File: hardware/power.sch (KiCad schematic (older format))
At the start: 49 parts, among them J4 USB_C_Receptacle, J5 Conn_01x01, J6 Conn_01x01, U10 TLV62568DBV, U2 TP4056, U4 XC6206P302MR, U7 TLV62568DBV, U8 TLV62568DBV, U9 TLV62568DBV

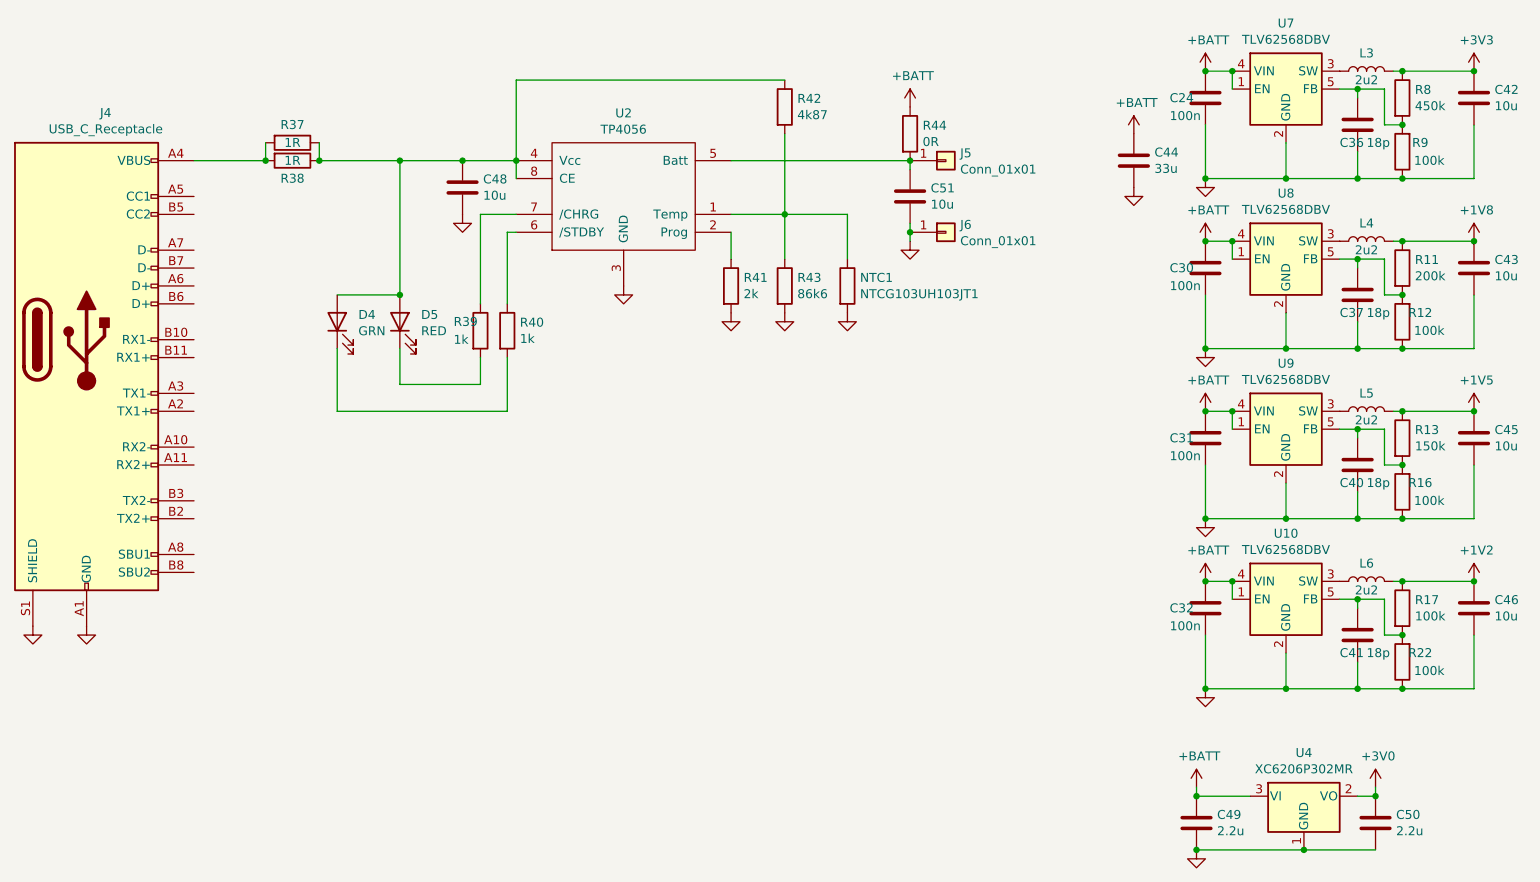
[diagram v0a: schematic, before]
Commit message: Power routing done
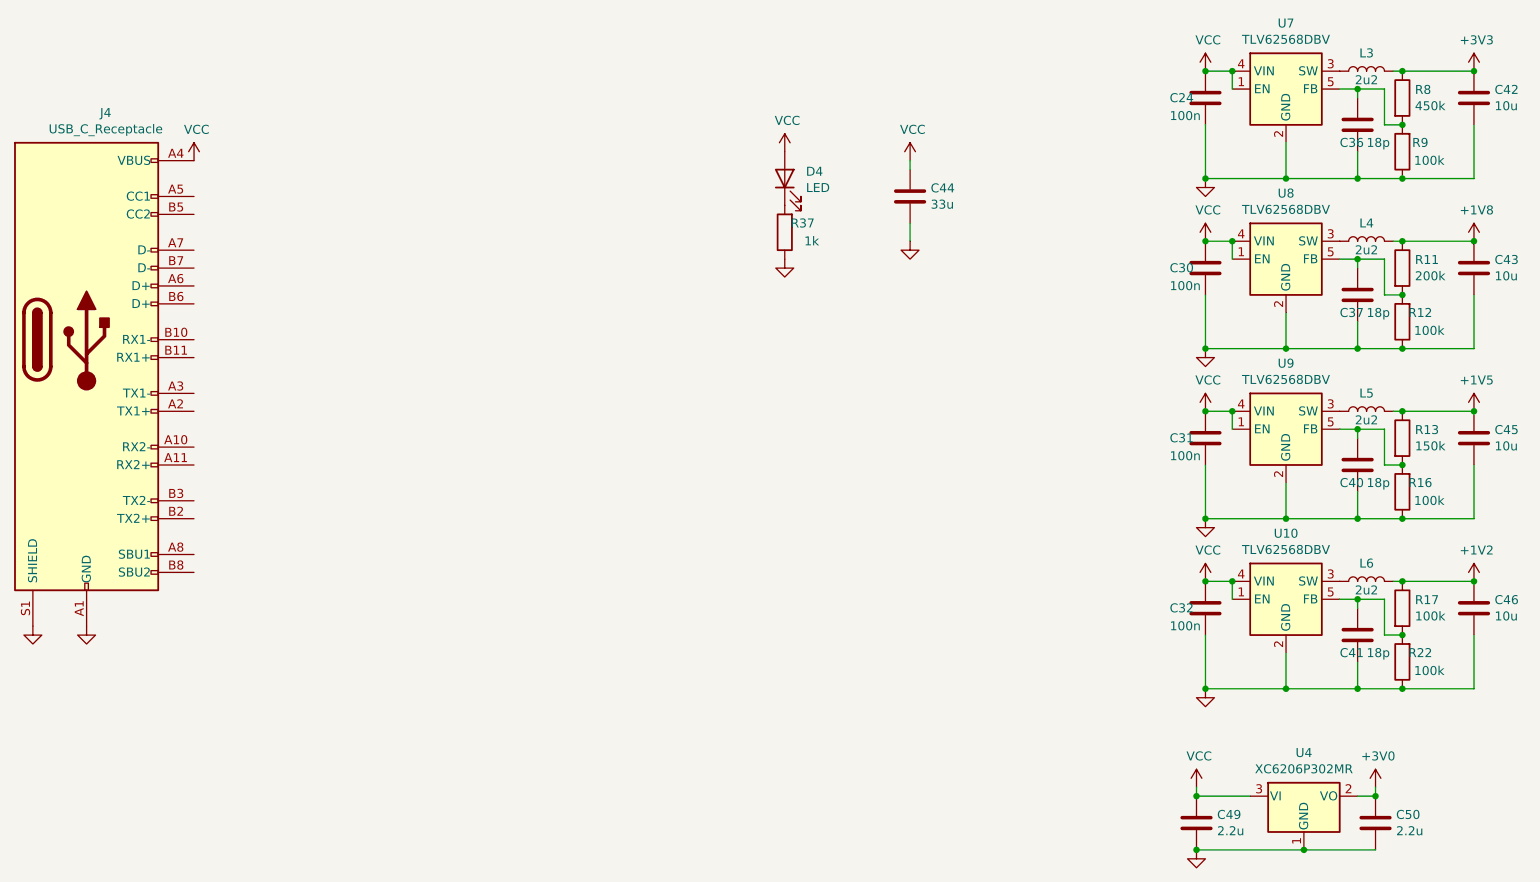
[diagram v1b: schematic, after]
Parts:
- removed C48, C51: 10u, Capacitor_SMD:C_0805_2012Metric, symbol Device:C
- removed D5: RED, LED_SMD:LED_0603_1608Metric, symbol Device:LED
- removed J5, J6: Conn_01x01, TestPoint:TestPoint_THTPad_1.0x1.0mm_Drill0.5mm, symbol Connector_Generic:Conn_01x01
- removed NTC1: NTCG103UH103JT1, Resistor_SMD:R_0603_1608Metric, symbol Device:R
- removed R38: 1R, Resistor_SMD:R_0603_1608Metric, symbol Device:R
- removed R39, R40: 1k, Resistor_SMD:R_0603_1608Metric, symbol Device:R
- removed R41: 2k, Resistor_SMD:R_0603_1608Metric, symbol Device:R
- removed R42: 4k87, Resistor_SMD:R_0603_1608Metric, symbol Device:R
- removed R43: 86k6, Resistor_SMD:R_0603_1608Metric, symbol Device:R
- removed R44: 0R, Resistor_SMD:R_0603_1608Metric, symbol Device:R
- removed U2: TP4056, Package_SO:SOP-8_3.9x4.9mm_P1.27mm, symbol custom:TP4056
- D4: value GRN -> LED
- R37: value 1R -> 1k
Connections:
- net +BATT is gone; now on net VCC: C24.1, C30.1, C31.1, C32.1, C44.1, C49.1, U10.1 (EN), U10.4 (VIN), U4.3 (VI), U7.1 (EN), U7.4 (VIN), U8.1 (EN), U8.4 (VIN), U9.1 (EN), U9.4 (VIN)
- net GND: now also R37.1
- net VCC: now reaches D4.2 (A)
- net VCC: now also J4.A4 (VBUS), J4.A9 (VBUS), J4.B4 (VBUS), J4.B9 (VBUS); no longer R37.1
- net at D4.1 (K): now also R37.2
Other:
- moved on the sheet: C44

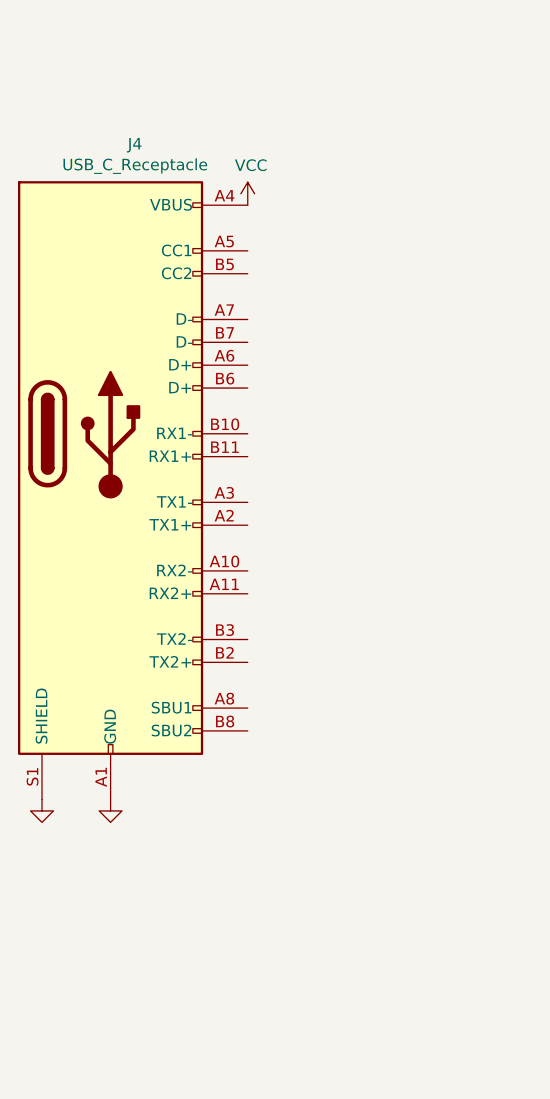
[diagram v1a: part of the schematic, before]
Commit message: Small touch-ups
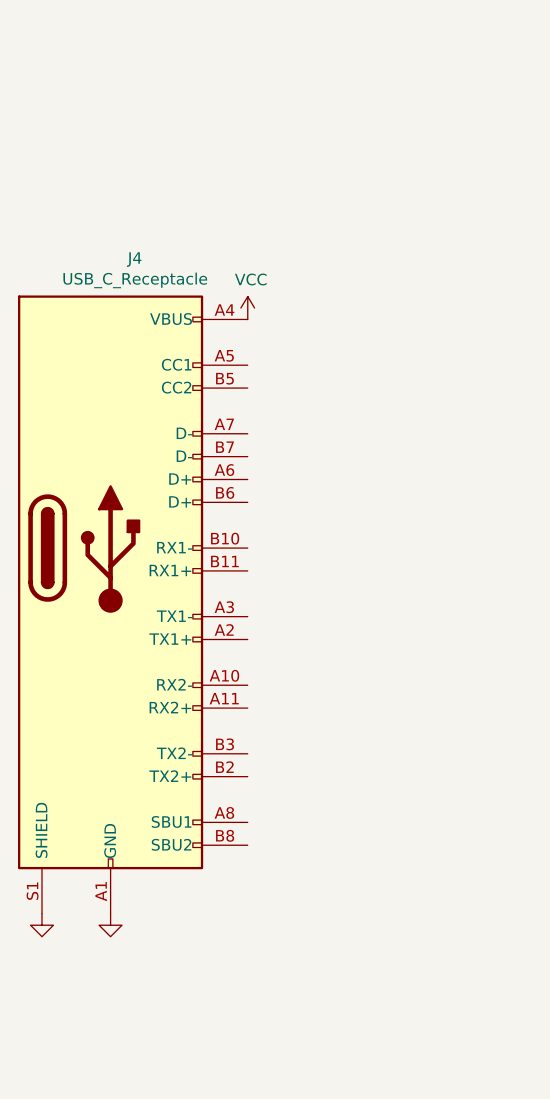
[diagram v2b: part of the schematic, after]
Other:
- moved on the sheet: J4
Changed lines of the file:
@@
 L Connector:USB_C_Receptacle J4
 U 1 1 6263C86C
-P 1150 2500
-F 0 "J4" H 1257 3767 50  0000 C CNN
-F 1 "USB_C_Receptacle" H 1257 3676 50  0000 C CNN
-F 2 "Connector_USB:USB_C_Receptacle_Amphenol_12401610E4-2A" H 1300 2500 50  0001 C CNN
-F 3 "https://www.usb.org/sites/default/files/documents/usb_type-c.zip" H 1300 2500 50  0001 C CNN
-	1    1150 2500
+P 1150 3000
+F 0 "J4" H 1257 4267 50  0000 C CNN
+F 1 "USB_C_Receptacle" H 1257 4176 50  0000 C CNN
+F 2 "Connector_USB:USB_C_Receptacle_Amphenol_12401610E4-2A" H 1300 3000 50  0001 C CNN
+F 3 "https://www.usb.org/sites/default/files/documents/usb_type-c.zip" H 1300 3000 50  0001 C CNN
+	1    1150 3000
 	1    0    0    -1
 $EndComp
@@
 L power:GND #PWR0138
 U 1 1 626D23B2
-P 1150 4100
-F 0 "#PWR0138" H 1150 3850 50  0001 C CNN
-F 1 "GND" H 1155 3927 50  0001 C CNN
-F 2 "" H 1150 4100 50  0001 C CNN
-F 3 "" H 1150 4100 50  0001 C CNN
-	1    1150 4100
+P 1150 4600
+F 0 "#PWR0138" H 1150 4350 50  0001 C CNN
+F 1 "GND" H 1155 4427 50  0001 C CNN
+F 2 "" H 1150 4600 50  0001 C CNN
+F 3 "" H 1150 4600 50  0001 C CNN
+	1    1150 4600
 	1    0    0    -1
 $EndComp
@@
 L power:GND #PWR0139
 U 1 1 626D2B67
-P 850 4100
-F 0 "#PWR0139" H 850 3850 50  0001 C CNN
-F 1 "GND" H 855 3927 50  0001 C CNN
-F 2 "" H 850 4100 50  0001 C CNN
-F 3 "" H 850 4100 50  0001 C CNN
-	1    850  4100
+P 850 4600
+F 0 "#PWR0139" H 850 4350 50  0001 C CNN
+F 1 "GND" H 855 4427 50  0001 C CNN
+F 2 "" H 850 4600 50  0001 C CNN
+F 3 "" H 850 4600 50  0001 C CNN
+	1    850  4600
 	1    0    0    -1
 $EndComp
@@
 L power:VCC #PWR0140
 U 1 1 625BC204
-P 1750 1500
-F 0 "#PWR0140" H 1750 1350 50  0001 C CNN
-F 1 "VCC" H 1765 1673 50  0000 C CNN
-F 2 "" H 1750 1500 50  0001 C CNN
-F 3 "" H 1750 1500 50  0001 C CNN
-	1    1750 1500
+P 1750 2000
+F 0 "#PWR0140" H 1750 1850 50  0001 C CNN
+F 1 "VCC" H 1765 2173 50  0000 C CNN
+F 2 "" H 1750 2000 50  0001 C CNN
+F 3 "" H 1750 2000 50  0001 C CNN
+	1    1750 2000
 	1    0    0    -1
 $EndComp
